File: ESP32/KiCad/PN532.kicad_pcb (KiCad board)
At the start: 2 copper layers, 42 x 42 mm, 33 parts, among them J1 Header, J2 SPOX, U1 PN532

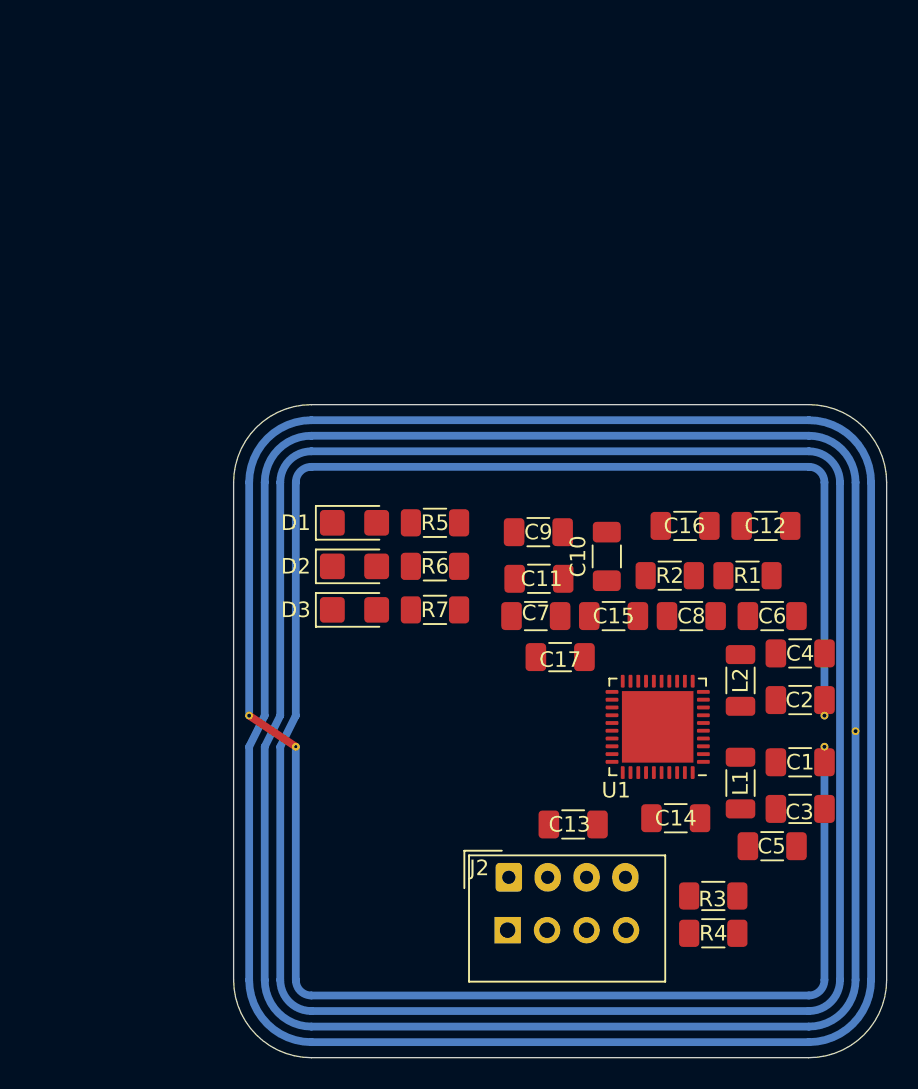
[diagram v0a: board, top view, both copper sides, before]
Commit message: Closer - not quite tracked yet
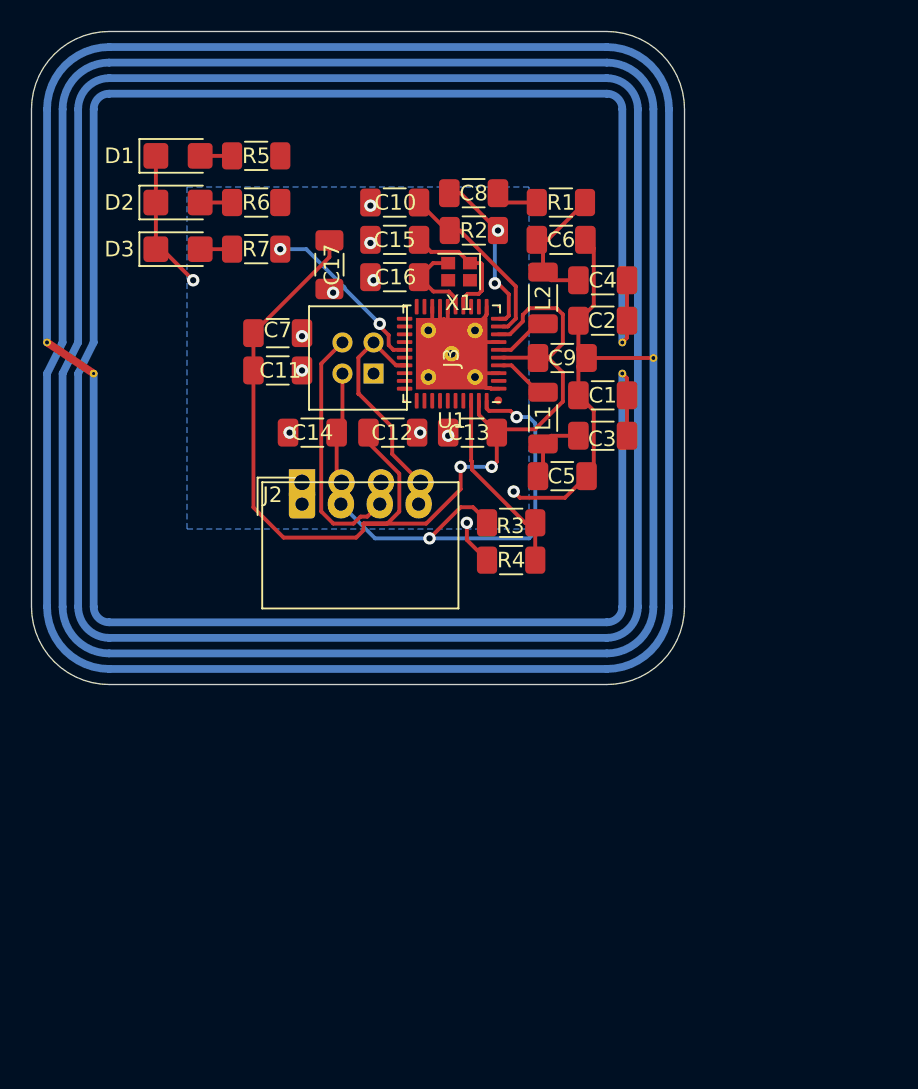
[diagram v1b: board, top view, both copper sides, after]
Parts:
- added J3: MiniGrid, RevK:Connector-MilliGrid-2x2, F.Cu at (121.0, 79.0)
- added X1: 27.12MHz, Crystal:Crystal_SMD_2016-4Pin_2.0x1.6mm, F.Cu at (127.5, 73.5)
- U1: footprint Package_DFN_QFN:QFN-40-1EP_6x6mm_P0.5mm_EP4.6x4.6mm -> RevK:QFN-40-(hand)-1EP_6x6mm_P0.5mm_EP4.6x4.6mm
- moved C14 34.1 mm to (118.1, 83.8), turned to 180 degrees
- moved J1 31.7 mm to (117.4, 87.0)
- moved C8 30.6 mm to (128.4, 68.4)
- moved C17 29.3 mm to (119.2, 73.0), turned to 270 degrees
- moved C15 28.0 mm to (123.4, 71.4), turned to 180 degrees
- moved C6 27.7 mm to (134.1, 71.4)
- moved L2 27.7 mm to (132.9, 75.1)
- moved C2 27.5 mm to (136.7, 76.6)
- moved J2 27.4 mm to (117.4, 88.4)
- moved U1 27.4 mm to (127.0, 78.7)
- moved C5 27.4 mm to (134.1, 86.6)
- moved A1 27.3 mm to (100.0, 58.0)
- moved R3 27.3 mm to (130.8, 89.6)
- moved R4 27.3 mm to (130.8, 92.0)
- moved C3 27.2 mm to (136.7, 84.0)
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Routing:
- net +3V3: track 0.00 -> 71.0 mm, vias 0 -> 2
- net GND: track 0.00 -> 68.8 mm, vias 0 -> 12
- net +5V: track 0.00 -> 38.3 mm, vias 0 -> 2
- net Net-(J1-Pad3): track 0.00 -> 16.4 mm
- net Net-(J1-Pad4): track 0.00 -> 14.2 mm
- net Net-(R3-Pad1): track 0.00 -> 12.3 mm
- net Net-(C10-Pad1): track 0.00 -> 11.6 mm
- net Net-(R7-Pad1): track 0.00 -> 11.2 mm, vias 0 -> 2
- net Net-(C8-Pad1): track 0.00 -> 10.9 mm, vias 0 -> 2
- net Net-(C4-Pad2): track 0.00 -> 8.83 mm
- net Net-(C15-Pad1): track 0.00 -> 8.34 mm
- net Net-(C16-Pad1): track 0.00 -> 5.71 mm
- net Net-(C3-Pad1): track 0.00 -> 4.70 mm
- net Net-(A1-Pad3): track 0.00 -> 4.12 mm
- net Net-(A1-Pad1): track 0.00 -> 4.12 mm
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- added copper zone on B.Cu, net GND
